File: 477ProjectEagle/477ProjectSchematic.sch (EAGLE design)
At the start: 67 parts, among them J1 POWER_JACK_BAT, J2 POWER_JACK_12VOUT, Q1 AO4419, X1 22-23-2051, X10 MOTORS, X2 XRJK-S-01-6-6-0-2G2-NO

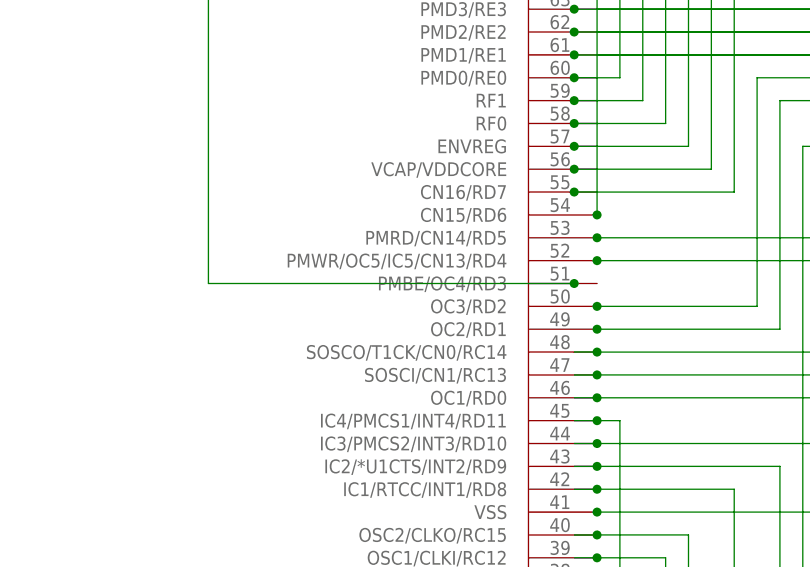
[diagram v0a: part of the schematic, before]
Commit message: minor changes to main PCB
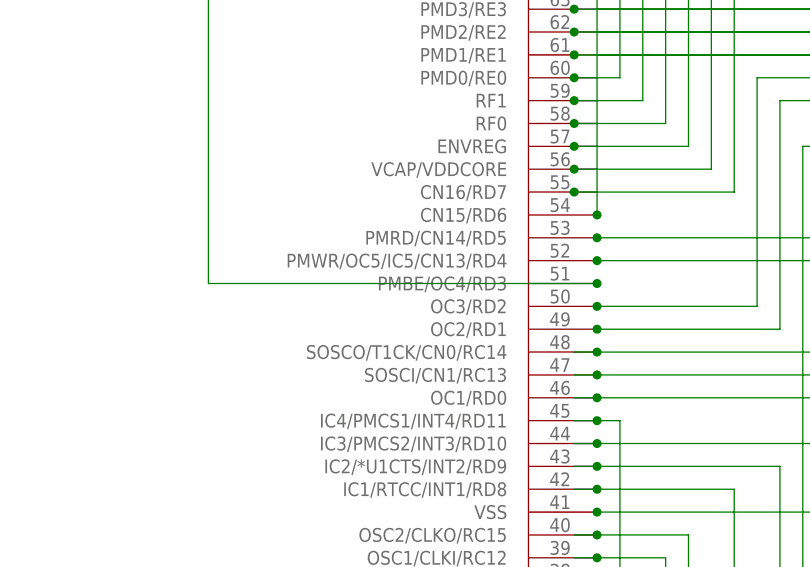
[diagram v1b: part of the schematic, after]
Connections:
- net N$85: now also U$1.PMBE/OC4/RD3
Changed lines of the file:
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@@
 <wire x1="91.44" y1="96.52" x2="33.02" y2="96.52" width="0.2032" layer="91"/>
 <wire x1="33.02" y1="96.52" x2="33.02" y2="15.24" width="0.2032" layer="91"/>
-<wire x1="33.02" y1="15.24" x2="73.66" y2="15.24" width="0.2032" layer="91"/>
-<junction x="73.66" y="15.24"/>
 <junction x="91.44" y="83.82"/>
+<pinref part="U$1" gate="A" pin="PMBE/OC4/RD3"/>
+<wire x1="33.02" y1="15.24" x2="76.2" y2="15.24" width="0.1524" layer="91"/>
+<junction x="76.2" y="15.24"/>
 </segment>
 </net>
